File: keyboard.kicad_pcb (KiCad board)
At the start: 2 copper layers, 228.6 x 76.2 mm, 232 parts, among them IC1 ATMEGA32U4, J1 USBMINI_B05, P1 ISP, P2 GPIO Port, Q1 MOS_P, X1 CRYSTAL

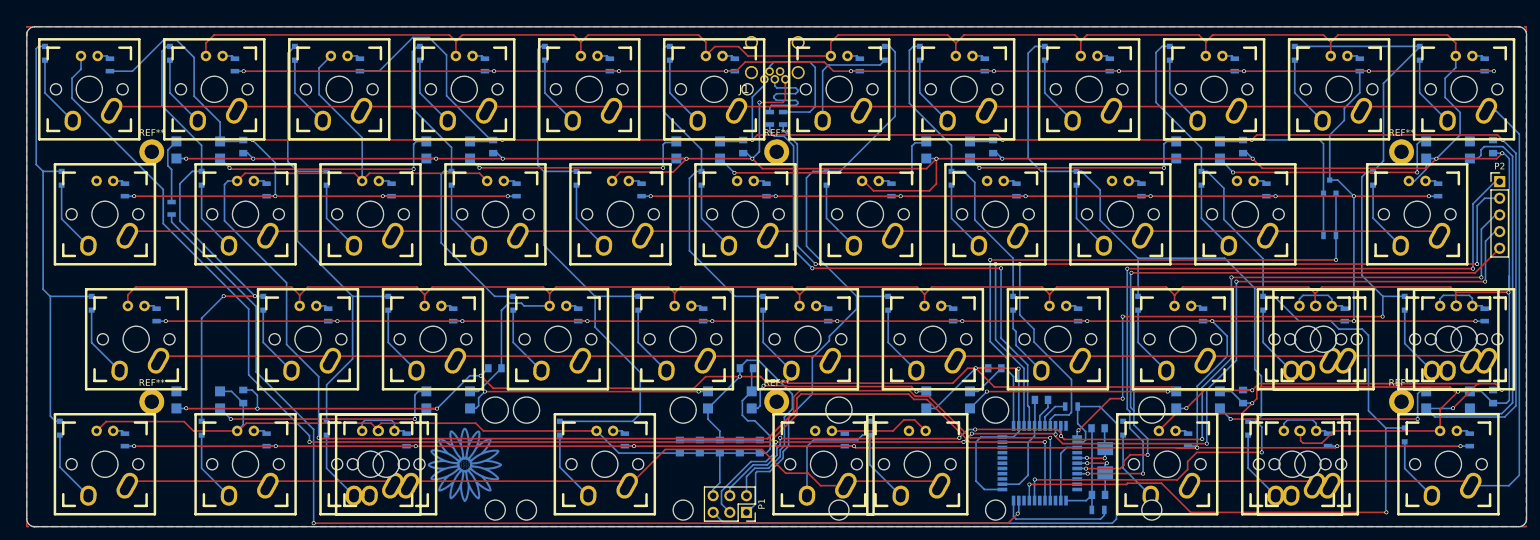
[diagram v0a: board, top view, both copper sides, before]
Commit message: Redesign v0.3
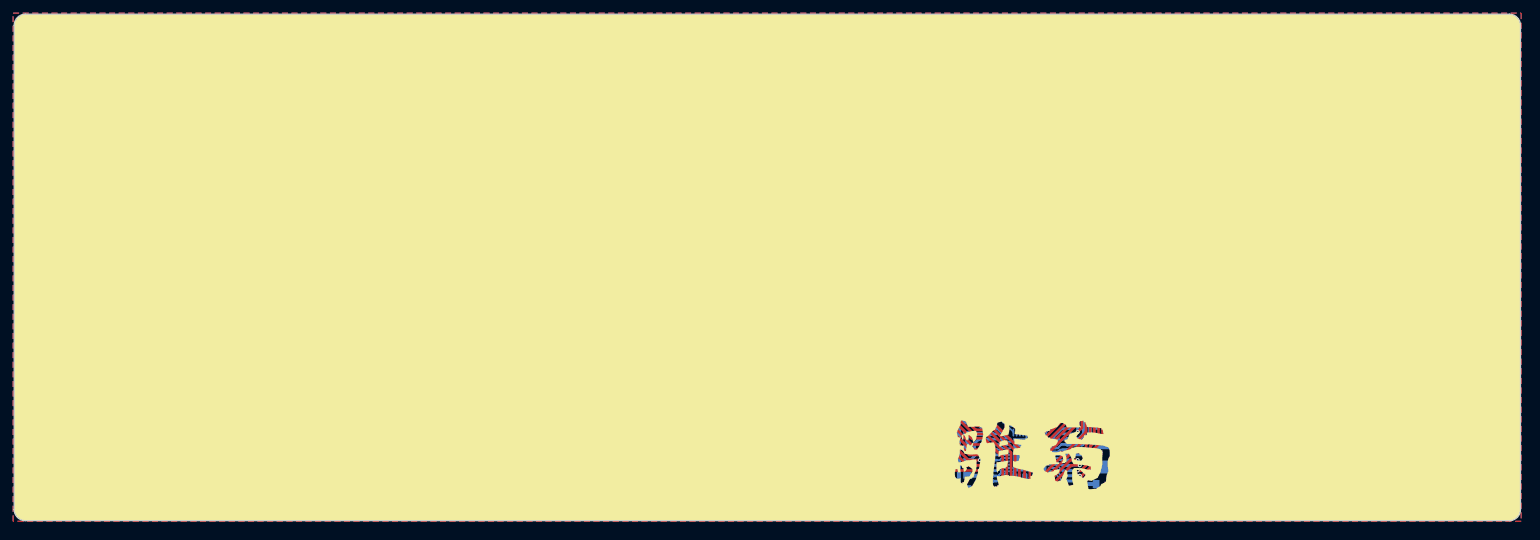
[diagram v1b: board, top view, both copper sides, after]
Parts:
- removed the C17 at (177.5, 82.0)
- removed the C18 at (139.7, 82.0)
- removed C19, C20: 100nF, Capacitors_SMD:C_0805
- removed the G*** at (96.8, 96.8) (x2)
- removed LED331, LED341, LED371, LED391, LED411: LED, mx1a:MX1A-led
- removed LR43: 330R, Resistors_SMD:R_0805
- removed R3: 10K, Resistors_SMD:R_0805
- removed RGBLED10, RGBLED11, RGBLED12, RGBLED9: WS2812B, WS2812B:WS2812B
- removed S321, S331, S361, S401: MX1A, keebs:Mx_Alps_100
- removed ktec-qr: , ktec:ktec-qr
- added ?: , ktec:THX2, B.Cu at (133.3, 95.2)
- added C10: 100nF, capacitors:C_0805, B.Cu at (173.4, 91.1)
- added C4: 100nF, capacitors:C_0805, B.Cu at (173.4, 95.2)
- added DA1: WE05-4RVLCH, diodes:SOT-23-6_Handsoldering, B.Cu at (142.9, 40.0)
- added JP1: JUMPER, passives:Jumper_SMD_2Pads_NC_V, B.Cu at (45.7, 38.1)
- added JP10: JUMPER, passives:Jumper_SMD_2Pads_NC_V, B.Cu at (55.9, 30.8)
- added JP11: JUMPER, passives:Jumper_SMD_2Pads_NC_V, B.Cu at (74.9, 30.8)
- added JP12: JUMPER, passives:Jumper_SMD_2Pads_NC_V, B.Cu at (94.0, 30.8)
- added JP13: JUMPER, passives:Jumper_SMD_2Pads_NC_V, B.Cu at (113.0, 30.8)
- added JP14: JUMPER, passives:Jumper_SMD_2Pads_NC_V, B.Cu at (132.1, 30.8)
- added JP15: JUMPER, passives:Jumper_SMD_2Pads_NC_V, B.Cu at (151.1, 30.8)
- added JP16: JUMPER, passives:Jumper_SMD_2Pads_NC_V, B.Cu at (170.2, 30.8)
- added JP17: JUMPER, passives:Jumper_SMD_2Pads_NC_V, B.Cu at (189.2, 30.8)
- added JP18: JUMPER, passives:Jumper_SMD_2Pads_NC_V, B.Cu at (208.3, 30.8)
- added JP19: JUMPER, passives:Jumper_SMD_2Pads_NC_V, B.Cu at (227.3, 30.8)
- added JP2: JUMPER, passives:Jumper_SMD_2Pads_NC_V, B.Cu at (51.4, 62.9)
- added JP3: JUMPER3, passives:Jumper_SMD_3Pads_NC12, B.Cu at (32.7, 32.1)
- added JP4: JUMPER3, passives:Jumper_SMD_3Pads_NC12, B.Cu at (35.1, 51.1)
- added JP5: JUMPER, passives:Jumper_SMD_2Pads_NC_V, B.Cu at (217.8, 36.8)
- added JP6: JUMPER, passives:Jumper_SMD_2Pads_NC_V, B.Cu at (222.6, 55.9)
- added JP7: JUMPER, passives:Jumper_SMD_2Pads_NC_V, B.Cu at (234.5, 74.9)
- added JP8: JUMPER, passives:Jumper_SMD_2Pads_NC_V, B.Cu at (253.5, 94.0)
- added JP9: JUMPER, passives:Jumper_SMD_2Pads_NC_V, B.Cu at (36.8, 30.8)
- added LED38: LED, leds:MX1A_LED_Polar, F.Cu at (164.3, 95.2)
- added LOGO1: , ktec:Daisy_Logo, B.Cu at (100.0, 94.3)
- added LOGO2: , ktec:Daisy_SilkS, F.Cu at (142.9, 66.7)
- added LR1-2: 330R, resistors:R_0805_NA, B.Cu at (43.8, 34.3)
- added LR12-2: 330R, resistors:R_0805_NA, B.Cu at (46.2, 53.3)
- added P3: GPIO_CLUSTER2, connectors:Socket_Strip_Straight_1x04_Pitch2.54mm, B.Cu at (29.2, 62.9)
- added R6: 4.7K, resistors:R_0805_NA, B.Cu at (34.4, 62.5)
- added R7: 4.7K, resistors:R_0805_NA, B.Cu at (46.5, 62.5)
- added REF**: Via_0.6mm, passives:Via_0.6mm, F.Cu at (127.6, 32.1)
- added SHIELD: Via_0.6mm, passives:Via_0.6mm, F.Cu at (241.6, 78.1)
- added SHIELD: Via_0.6mm, passives:Via_0.6mm, F.Cu at (123.2, 63.2)
- added SHIELD: Via_0.6mm, passives:Via_0.6mm, F.Cu at (70.5, 32.1)
- added SHIELD: Via_0.6mm, passives:Via_0.6mm, F.Cu at (89.5, 32.1)
- added SHIELD: Via_0.6mm, passives:Via_0.6mm, F.Cu at (108.6, 32.1)
- added SHIELD: Via_0.6mm, passives:Via_0.6mm, F.Cu at (165.7, 32.1)
- added SHIELD: Via_0.6mm, passives:Via_0.6mm, F.Cu at (104.1, 63.2)
- added SHIELD: Via_0.6mm, passives:Via_0.6mm, F.Cu at (85.1, 63.2)
- added SHIELD: Via_0.6mm, passives:Via_0.6mm, F.Cu at (66.0, 63.2)
- added SHIELD: Via_0.6mm, passives:Via_0.6mm, F.Cu at (44.1, 63.2)
- added SHIELD: Via_0.6mm, passives:Via_0.6mm, F.Cu at (212.7, 44.8)
- added SHIELD: Via_0.6mm, passives:Via_0.6mm, F.Cu at (193.7, 44.8)
- added SHIELD: Via_0.6mm, passives:Via_0.6mm, F.Cu at (174.6, 44.8)
- added SHIELD: Via_0.6mm, passives:Via_0.6mm, F.Cu at (155.6, 44.8)
- added SHIELD: Via_0.6mm, passives:Via_0.6mm, F.Cu at (117.8, 44.5)
- added SHIELD: Via_0.6mm, passives:Via_0.6mm, F.Cu at (217.5, 97.2)
- added SHIELD: Via_0.6mm, passives:Via_0.6mm, F.Cu at (98.4, 44.8)
- added SHIELD: Via_0.6mm, passives:Via_0.6mm, F.Cu at (79.4, 44.8)
- added SHIELD: Via_0.6mm, passives:Via_0.6mm, F.Cu at (60.3, 44.8)
- added SHIELD: Via_0.6mm, passives:Via_0.6mm, F.Cu at (157.8, 88.6)
- added SHIELD: Via_0.6mm, passives:Via_0.6mm, F.Cu at (208.3, 86.4)
- added SHIELD: Via_0.6mm, passives:Via_0.6mm, F.Cu at (207.3, 93.7)
- added SHIELD: Via_0.6mm, passives:Via_0.6mm, F.Cu at (199.7, 78.7)
- added SHIELD: Via_0.6mm, passives:Via_0.6mm, F.Cu at (157.2, 95.2)
- added SHIELD: Via_0.6mm, passives:Via_0.6mm, F.Cu at (77.2, 97.2)
- added SHIELD: Via_0.6mm, passives:Via_0.6mm, F.Cu at (128.6, 79.4)
- added SHIELD: Via_0.6mm, passives:Via_0.6mm, F.Cu at (151.8, 81.6)
- added SHIELD: Via_0.6mm, passives:Via_0.6mm, F.Cu at (208.3, 74.6)
- added SHIELD: Via_0.6mm, passives:Via_0.6mm, F.Cu at (220.0, 78.1)
- added SHIELD: Via_0.6mm, passives:Via_0.6mm, F.Cu at (218.8, 80.3)
- added SHIELD: Via_0.6mm, passives:Via_0.6mm, F.Cu at (216.2, 80.6)
- added SHIELD: Via_0.6mm, passives:Via_0.6mm, F.Cu at (161.0, 63.2)
- added SHIELD: Via_0.6mm, passives:Via_0.6mm, F.Cu at (218.1, 70.2)
- added SHIELD: Via_0.6mm, passives:Via_0.6mm, F.Cu at (212.4, 71.4)
- added SHIELD: Via_0.6mm, passives:Via_0.6mm, F.Cu at (231.1, 82.5)
- added SHIELD: Via_0.6mm, passives:Via_0.6mm, F.Cu at (239.7, 80.3)
- added SHIELD: Via_0.6mm, passives:Via_0.6mm, F.Cu at (239.4, 70.2)
- added SHIELD: Via_0.6mm, passives:Via_0.6mm, F.Cu at (66.4, 81.6)
- added SHIELD: Via_0.6mm, passives:Via_0.6mm, F.Cu at (122.9, 82.2)
- added SHIELD: Via_0.6mm, passives:Via_0.6mm, F.Cu at (32.7, 62.5)
- added SHIELD: Via_0.6mm, passives:Via_0.6mm, F.Cu at (236.2, 53.3)
- added SHIELD: Via_0.6mm, passives:Via_0.6mm, F.Cu at (48.3, 52.4)
- added SHIELD: Via_0.6mm, passives:Via_0.6mm, F.Cu at (48.9, 55.9)
- added SHIELD: Via_0.6mm, passives:Via_0.6mm, F.Cu at (40.3, 63.2)
- added SHIELD: Via_0.6mm, passives:Via_0.6mm, F.Cu at (57.1, 51.1)
- added SHIELD: Via_0.6mm, passives:Via_0.6mm, F.Cu at (114.3, 43.5)
- added SHIELD: Via_0.6mm, passives:Via_0.6mm, F.Cu at (180.7, 78.7)
- added SHIELD: Via_0.6mm, passives:Via_0.6mm, F.Cu at (189.9, 74.3)
- added SHIELD: Via_0.6mm, passives:Via_0.6mm, F.Cu at (40.6, 85.1)
- added SHIELD: Via_0.6mm, passives:Via_0.6mm, F.Cu at (203.5, 102.2)
- added SHIELD: Via_0.6mm, passives:Via_0.6mm, F.Cu at (215.9, 89.2)
- added SHIELD: Via_0.6mm, passives:Via_0.6mm, F.Cu at (247.3, 85.7)
- added SHIELD: Via_0.6mm, passives:Via_0.6mm, F.Cu at (161.6, 78.7)
- added SHIELD: Via_0.6mm, passives:Via_0.6mm, F.Cu at (84.8, 82.5)
- added SHIELD: Via_0.6mm, passives:Via_0.6mm, F.Cu at (73.7, 89.2)
- added SHIELD: Via_0.6mm, passives:Via_0.6mm, F.Cu at (43.5, 43.5)
- added SHIELD: Via_0.6mm, passives:Via_0.6mm, F.Cu at (39.1, 47.6)
- added SHIELD: Via_0.6mm, passives:Via_0.6mm, F.Cu at (58.7, 76.2)
- added SHIELD: Via_0.6mm, passives:Via_0.6mm, F.Cu at (100.0, 76.2)
- added SHIELD: Via_0.6mm, passives:Via_0.6mm, F.Cu at (244.8, 63.2)
- added SHIELD: Via_0.6mm, passives:Via_0.6mm, F.Cu at (119.1, 76.2)
- added SHIELD: Via_0.6mm, passives:Via_0.6mm, F.Cu at (138.1, 76.2)
- added SHIELD: Via_0.6mm, passives:Via_0.6mm, F.Cu at (134.0, 87.9)
- added SHIELD: Via_0.6mm, passives:Via_0.6mm, F.Cu at (109.9, 88.6)
- added SHIELD: Via_0.6mm, passives:Via_0.6mm, F.Cu at (254.0, 101.9)
- added SHIELD: Via_0.6mm, passives:Via_0.6mm, F.Cu at (31.8, 101.9)
- added SHIELD: Via_0.6mm, passives:Via_0.6mm, F.Cu at (144.8, 61.3)
- added SHIELD: Via_0.6mm, passives:Via_0.6mm, F.Cu at (138.1, 63.5)
- added SHIELD: Via_0.6mm, passives:Via_0.6mm, F.Cu at (161.0, 70.2)
- added SHIELD: Via_0.6mm, passives:Via_0.6mm, F.Cu at (157.2, 62.9)
- added SHIELD: Via_0.6mm, passives:Via_0.6mm, F.Cu at (199.4, 63.2)
- added SHIELD: Via_0.6mm, passives:Via_0.6mm, F.Cu at (218.4, 63.2)
- added SHIELD: Via_0.6mm, passives:Via_0.6mm, F.Cu at (222.6, 61.6)
- added SHIELD: Via_0.6mm, passives:Via_0.6mm, F.Cu at (227.3, 56.8)
- added SHIELD: Via_0.6mm, passives:Via_0.6mm, F.Cu at (185.7, 57.1)
- added SHIELD: Via_0.6mm, passives:Via_0.6mm, F.Cu at (166.7, 57.1)
- added SHIELD: Via_0.6mm, passives:Via_0.6mm, F.Cu at (141.9, 70.2)
- added SHIELD: Via_0.6mm, passives:Via_0.6mm, F.Cu at (34.6, 73.3)
- added SHIELD: Via_0.6mm, passives:Via_0.6mm, F.Cu at (32.7, 54.3)
- added SHIELD: Via_0.6mm, passives:Via_0.6mm, F.Cu at (56.5, 61.0)
- added SHIELD: Via_0.6mm, passives:Via_0.6mm, F.Cu at (71.4, 57.1)
- added SHIELD: Via_0.6mm, passives:Via_0.6mm, F.Cu at (180.3, 63.2)
- added SHIELD: Via_0.6mm, passives:Via_0.6mm, F.Cu at (90.5, 57.1)
- added SHIELD: Via_0.6mm, passives:Via_0.6mm, F.Cu at (109.5, 57.1)
- added SHIELD: Via_0.6mm, passives:Via_0.6mm, F.Cu at (128.6, 57.1)
- added SHIELD: Via_0.6mm, passives:Via_0.6mm, F.Cu at (139.1, 42.5)
- added SHIELD: Via_0.6mm, passives:Via_0.6mm, F.Cu at (136.5, 45.1)
- added SHIELD: Via_0.6mm, passives:Via_0.6mm, F.Cu at (146.7, 42.5)
- added SHIELD: Via_0.6mm, passives:Via_0.6mm, F.Cu at (113.0, 51.1)
- added SHIELD: Via_0.6mm, passives:Via_0.6mm, F.Cu at (132.1, 51.1)
- added SHIELD: Via_0.6mm, passives:Via_0.6mm, F.Cu at (246.4, 48.6)
- added SHIELD: Via_0.6mm, passives:Via_0.6mm, F.Cu at (253.4, 56.2)
- added SHIELD: Via_0.6mm, passives:Via_0.6mm, F.Cu at (142.2, 63.2)
- added SHIELD: Via_0.6mm, passives:Via_0.6mm, F.Cu at (224.8, 51.1)
- added SHIELD: Via_0.6mm, passives:Via_0.6mm, F.Cu at (234.9, 44.1)
- added SHIELD: Via_0.6mm, passives:Via_0.6mm, F.Cu at (189.2, 51.1)
- added SHIELD: Via_0.6mm, passives:Via_0.6mm, F.Cu at (104.8, 38.1)
- added SHIELD: Via_0.6mm, passives:Via_0.6mm, F.Cu at (161.9, 38.1)
- added SHIELD: Via_0.6mm, passives:Via_0.6mm, F.Cu at (123.8, 38.1)
- added SHIELD: Via_0.6mm, passives:Via_0.6mm, F.Cu at (222.9, 32.1)
- added SHIELD: Via_0.6mm, passives:Via_0.6mm, F.Cu at (203.8, 32.1)
- added SHIELD: Via_0.6mm, passives:Via_0.6mm, F.Cu at (184.8, 32.1)
- added SHIELD: Via_0.6mm, passives:Via_0.6mm, F.Cu at (51.4, 32.1)
- C1, C2, C3: footprint Capacitors_SMD:C_0805 -> capacitors:C_0805
- C11: renamed from C9; footprint Capacitors_SMD:C_0805 -> capacitors:C_0805_V2
- C12: renamed from C10; footprint Capacitors_SMD:C_0805 -> capacitors:C_0805_V2
- C13: renamed from C11; footprint Capacitors_SMD:C_0805 -> capacitors:C_0805_V2
- C14: renamed from C12; footprint Capacitors_SMD:C_0805 -> capacitors:C_0805_V1
- C15: renamed from C13; footprint Capacitors_SMD:C_0805 -> capacitors:C_0805_V1
- C16: renamed from C14; footprint Capacitors_SMD:C_0805 -> capacitors:C_0805_V1
- C17: renamed from C15; footprint Capacitors_SMD:C_0805 -> capacitors:C_0805_V1
- C18: renamed from C16; footprint Capacitors_SMD:C_0805 -> capacitors:C_0805_V2
- C5: renamed from C8; footprint Capacitors_SMD:C_0805 -> capacitors:C_0805
- C6: renamed from C4; footprint Capacitors_SMD:C_0805 -> capacitors:C_0805
- C7: renamed from C5; footprint Capacitors_SMD:C_0805 -> capacitors:C_0805
- C8: renamed from C6; footprint Capacitors_SMD:C_0805 -> capacitors:C_0805
- C9: renamed from C7; footprint Capacitors_SMD:C_0805 -> capacitors:C_0805
- D1, D10, D11, D12, D13, D14, D15, D16, D17, D18, D19, D2, D20, D21, D22, D23, D24, D25, D26, D27, D28, D29, D3, D30, D31, D32, D33, D34, D35, D36, D37, D38, D39, D4, D40, D41, D42, D5, D6, D7, D8, D9: footprint Diodes_SMD:D_0805 -> diodes:D_0805_V2
- J1: value USBMINI_B05 -> USB_MINI-B; footprint USB:DX_USB -> connectors:USB_MINI-B
- LED1, LED10, LED11, LED12, LED13, LED14, LED15, LED16, LED17, LED18, LED19, LED2, LED20, LED21, LED22, LED23, LED24, LED25, LED26, LED27, LED28, LED29, LED3, LED30, LED31, LED34, LED35, LED37, LED39, LED4, LED41, LED42, LED5, LED6, LED7, LED8, LED9: footprint mx1a:MX1A-led -> leds:MX1A_LED_Polar
- LED32, LED33, LED36, LED40: footprint mx1a:MX1A-led -> leds:MX1A_LED_Polar_Dual
- LED38_625: renamed from LED38; footprint mx1a:MX1A-led -> leds:MX1A_LED_Polar
- LR1, LR10, LR11, LR12, LR13, LR14, LR15, LR16, LR17, LR18, LR19, LR2, LR20, LR21, LR22, LR23, LR24, LR25, LR26, LR27, LR28, LR29, LR3, LR30, LR31, LR32, LR33, LR34, LR35, LR36, LR37, LR38, LR39, LR4, LR40, LR41, LR42, LR5, LR6, LR7, LR8, LR9, R1, R2: footprint Resistors_SMD:R_0805 -> resistors:R_0805_V1
- P1: footprint Socket_Strips:Socket_Strip_Straight_2x03_Pitch2.54mm -> connectors:Socket_Strip_Straight_1x06_Pitch2.54mm; moved to B.Cu
- P2: value GPIO Port -> GPIO_CLUSTER1; footprint Socket_Strips:Socket_Strip_Straight_1x05_Pitch2.54mm -> connectors:Socket_Strip_Straight_2x04_Pitch2.54mm; moved to B.Cu
- Q1: footprint SI2305:SOT-23 -> transistors:SOT-23
- R4, R5: footprint Resistors_SMD:R_0805 -> resistors:R_0805
- RGBLED1, RGBLED2, RGBLED3, RGBLED4, RGBLED5, RGBLED6, RGBLED7, RGBLED8: footprint WS2812B:WS2812B -> leds:WS2812B
- SW1: renamed from S1; footprint keebs:Mx_Alps_100 -> switches:Mx_Alps_100_NoFSilk
- SW10: renamed from S10; footprint keebs:Mx_Alps_100 -> switches:Mx_Alps_100_NoFSilk
- SW11: renamed from S11; footprint keebs:Mx_Alps_100 -> switches:Mx_Alps_100_NoFSilk
- SW12: renamed from S12; footprint keebs:Mx_Alps_100 -> switches:Mx_Alps_125_NoFSilk
- SW13: renamed from S13; footprint keebs:Mx_Alps_100 -> switches:Mx_Alps_100_NoFSilk
- SW14: renamed from S14; footprint keebs:Mx_Alps_100 -> switches:Mx_Alps_100_NoFSilk
- SW15: renamed from S15; footprint keebs:Mx_Alps_100 -> switches:Mx_Alps_100_NoFSilk
- SW16: renamed from S16; footprint keebs:Mx_Alps_100 -> switches:Mx_Alps_100_NoFSilk
- SW17: renamed from S17; footprint keebs:Mx_Alps_100 -> switches:Mx_Alps_100_NoFSilk
- SW18: renamed from S18; footprint keebs:Mx_Alps_100 -> switches:Mx_Alps_100_NoFSilk
- SW19: renamed from S19; footprint keebs:Mx_Alps_100 -> switches:Mx_Alps_100_NoFSilk
- SW2: renamed from S2; footprint keebs:Mx_Alps_100 -> switches:Mx_Alps_100_NoFSilk
- SW20: renamed from S20; footprint keebs:Mx_Alps_100 -> switches:Mx_Alps_100_NoFSilk
- SW21: renamed from S21; footprint keebs:Mx_Alps_100 -> switches:Mx_Alps_100_NoFSilk
- SW22: renamed from S22; footprint keebs:Mx_Alps_100 -> switches:Mx_Alps_175_NoFSilk
- SW23: renamed from S23; footprint keebs:Mx_Alps_100 -> switches:Mx_Alps_175_NoFSilk
- SW24: renamed from S24; footprint keebs:Mx_Alps_100 -> switches:Mx_Alps_100_NoFSilk
- SW25: renamed from S25; footprint keebs:Mx_Alps_100 -> switches:Mx_Alps_100_NoFSilk
- SW26: renamed from S26; footprint keebs:Mx_Alps_100 -> switches:Mx_Alps_100_NoFSilk
- SW27: renamed from S27; footprint keebs:Mx_Alps_100 -> switches:Mx_Alps_100_NoFSilk
- SW28: renamed from S28; footprint keebs:Mx_Alps_100 -> switches:Mx_Alps_100_NoFSilk
- SW29: renamed from S29; footprint keebs:Mx_Alps_100 -> switches:Mx_Alps_100_NoFSilk
- SW3: renamed from S3; footprint keebs:Mx_Alps_100 -> switches:Mx_Alps_100_NoFSilk
- SW30: renamed from S30; footprint keebs:Mx_Alps_100 -> switches:Mx_Alps_100_NoFSilk
- SW31: renamed from S31; footprint keebs:Mx_Alps_100 -> switches:Mx_Alps_100_NoFSilk
- SW32: renamed from S32; footprint keebs:Mx_Alps_100 -> switches:Mx_Alps_100_Dual_NoFSilk
- SW33: renamed from S33; footprint keebs:Mx_Alps_100 -> switches:Mx_Alps_100_Dual_NoFSilk
- SW34: renamed from S34; footprint keebs:Mx_Alps_100 -> switches:Mx_Alps_125_NoFSilk
- SW35: renamed from S35; footprint keebs:Mx_Alps_100 -> switches:Mx_Alps_100_NoFSilk
- SW36: renamed from S36; footprint keebs:Mx_Alps_100 -> switches:Mx_Alps_100_Dual_NoFSilk
- SW37: renamed from S37; footprint keebs:Mx_Alps_225 -> switches:Mx_Alps_225_NoFSilk
- SW38: renamed from S381; footprint keebs:Mx_Alps_275 -> switches:Mx_Alps_275_NoFSilk
- SW38_625: renamed from S38; footprint keebs:Mx_Alps_625 -> switches:Mx_Alps_625_NoFSilk
- SW39: renamed from S39; footprint keebs:Mx_Alps_100 -> switches:Mx_Alps_100_NoFSilk
- SW4: renamed from S4; footprint keebs:Mx_Alps_100 -> switches:Mx_Alps_100_NoFSilk
- SW40: renamed from S40; footprint keebs:Mx_Alps_100 -> switches:Mx_Alps_100_Dual_NoFSilk
- SW41: renamed from S41; footprint keebs:Mx_Alps_100 -> switches:Mx_Alps_125_NoFSilk
- SW42: renamed from S42; footprint keebs:Mx_Alps_100 -> switches:Mx_Alps_100_NoFSilk
- SW5: renamed from S5; footprint keebs:Mx_Alps_100 -> switches:Mx_Alps_100_NoFSilk
- SW6: renamed from S6; footprint keebs:Mx_Alps_100 -> switches:Mx_Alps_100_NoFSilk
- SW7: renamed from S7; footprint keebs:Mx_Alps_100 -> switches:Mx_Alps_100_NoFSilk
- SW8: renamed from S8; footprint keebs:Mx_Alps_100 -> switches:Mx_Alps_100_NoFSilk
- SW9: renamed from S9; footprint keebs:Mx_Alps_100 -> switches:Mx_Alps_100_NoFSilk
- U1: renamed from IC1; footprint Housings_QFP:TQFP-44_10x10mm_Pitch0.8mm -> housings:TQFP44+QFN44
- moved LED34 209.3 mm to (40.5, 95.2)
- moved LR34 206.8 mm to (46.2, 91.4), turned to 270 degrees
- moved LED23 197.5 mm to (45.2, 76.2)
- moved LR23 194.9 mm to (51.0, 72.4), turned to 270 degrees
- moved LR11 190.5 mm to (234.3, 34.3), turned to 270 degrees
- moved LED11 187.8 mm to (228.6, 38.1)
- moved Q1 177.2 mm to (51.4, 57.1)
- moved R4 177.2 mm to (51.4, 60.3)
- moved RGBLED1 118.1 mm to (168.3, 85.7), turned to 0 degrees
- moved C11 106.7 mm to (162.9, 85.7)
- moved C14 105.2 mm to (72.1, 47.6), turned to 270 degrees
- moved RGBLED4 103.8 mm to (66.7, 47.6)
- moved C15 92.5 mm to (122.9, 47.6), turned to 270 degrees
- moved RGBLED5 91.1 mm to (117.5, 47.6)
- moved C16 90.6 mm to (162.9, 47.6), turned to 270 degrees
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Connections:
- net /~Res renamed /~RESET
- C11 pad 1: GND -> VCC
- C11 pad 2: VCC -> GND
- C12 pad 1: GND -> VCC
- C12 pad 2: VCC -> GND
- C13 pad 1: GND -> VCC
- C13 pad 2: VCC -> GND
- C14 pad 1: GND -> VCC
- C14 pad 2: VCC -> GND
- C15 pad 1: GND -> VCC
- C15 pad 2: VCC -> GND
- C16 pad 1: GND -> VCC
- C16 pad 2: VCC -> GND
- C17 pad 1: GND -> VCC
- C17 pad 2: VCC -> GND
- C18 pad 1: GND -> VCC
- C18 pad 2: VCC -> GND
- D1 pad 1: /Col0 -> Net-(D1-Pad1)
- D1 pad 2: Net-(D1-Pad2) -> /matrix/Row0
- D10 pad 1: /Col9 -> Net-(D10-Pad1)
- D10 pad 2: Net-(D10-Pad2) -> /matrix/Row0
- D11 pad 1: /Col10 -> Net-(D11-Pad1)
- D11 pad 2: Net-(D11-Pad2) -> /matrix/Row0
- D12 pad 1: /Col0 -> Net-(D12-Pad1)
- D12 pad 2: Net-(D12-Pad2) -> /matrix/Row1
- D13 pad 1: /Col1 -> Net-(D13-Pad1)
- D13 pad 2: Net-(D13-Pad2) -> /matrix/Row1
- D14 pad 1: /Col2 -> Net-(D14-Pad1)
- D14 pad 2: Net-(D14-Pad2) -> /matrix/Row1
- D15 pad 1: /Col3 -> Net-(D15-Pad1)
- D15 pad 2: Net-(D15-Pad2) -> /matrix/Row1
- D16 pad 1: /Col4 -> Net-(D16-Pad1)
- D16 pad 2: Net-(D16-Pad2) -> /matrix/Row1
- D17 pad 1: /Col5 -> Net-(D17-Pad1)
- D17 pad 2: Net-(D17-Pad2) -> /matrix/Row1
- D18 pad 1: /Col6 -> Net-(D18-Pad1)
- D18 pad 2: Net-(D18-Pad2) -> /matrix/Row1
- D19 pad 1: /Col7 -> Net-(D19-Pad1)
- D19 pad 2: Net-(D19-Pad2) -> /matrix/Row1
- D2 pad 1: /Col1 -> Net-(D2-Pad1)
- D2 pad 2: Net-(D2-Pad2) -> /matrix/Row0
- D20 pad 1: /Col8 -> Net-(D20-Pad1)
- D20 pad 2: Net-(D20-Pad2) -> /matrix/Row1
- D21 pad 1: /Col9 -> Net-(D21-Pad1)
- D21 pad 2: Net-(D21-Pad2) -> /matrix/Row1
- D22 pad 1: /Col10 -> Net-(D22-Pad1)
- D22 pad 2: Net-(D22-Pad2) -> /matrix/Row1
- D23 pad 1: /Col0 -> Net-(D23-Pad1)
- D23 pad 2: Net-(D23-Pad2) -> /matrix/Row2
- D24 pad 1: /Col1 -> Net-(D24-Pad1)
- D24 pad 2: Net-(D24-Pad2) -> /matrix/Row2
- D25 pad 1: /Col2 -> Net-(D25-Pad1)
- D25 pad 2: Net-(D25-Pad2) -> /matrix/Row2
- D26 pad 1: /Col3 -> Net-(D26-Pad1)
- D26 pad 2: Net-(D26-Pad2) -> /matrix/Row2
- D27 pad 1: /Col4 -> Net-(D27-Pad1)
- D27 pad 2: Net-(D27-Pad2) -> /matrix/Row2
- D28 pad 1: /Col5 -> Net-(D28-Pad1)
- D28 pad 2: Net-(D28-Pad2) -> /matrix/Row2
- D29 pad 1: /Col6 -> Net-(D29-Pad1)
- D29 pad 2: Net-(D29-Pad2) -> /matrix/Row2
- D3 pad 1: /Col2 -> Net-(D3-Pad1)
- D3 pad 2: Net-(D3-Pad2) -> /matrix/Row0
- D30 pad 1: /Col7 -> Net-(D30-Pad1)
- D30 pad 2: Net-(D30-Pad2) -> /matrix/Row2
- D31 pad 1: /Col8 -> Net-(D31-Pad1)
- D31 pad 2: Net-(D31-Pad2) -> /matrix/Row2
- D32 pad 1: /Col9 -> Net-(D32-Pad1)
- D32 pad 2: Net-(D32-Pad2) -> /matrix/Row2
- D33 pad 1: /Col10 -> Net-(D33-Pad1)
- D33 pad 2: Net-(D33-Pad2) -> /matrix/Row2
- D34 pad 1: /Col0 -> Net-(D34-Pad1)
- D34 pad 2: Net-(D34-Pad2) -> /matrix/Row3
- D35 pad 1: /Col1 -> Net-(D35-Pad1)
- D35 pad 2: Net-(D35-Pad2) -> /matrix/Row3
- D36 pad 1: /Col2 -> Net-(D36-Pad1)
- D36 pad 2: Net-(D36-Pad2) -> /matrix/Row3
- D37 pad 1: /Col4 -> Net-(D37-Pad1)
- D37 pad 2: Net-(D37-Pad2) -> /matrix/Row3
- D38 pad 1: /Col5 -> Net-(D38-Pad1)
- D38 pad 2: Net-(D38-Pad2) -> /matrix/Row3
- D39 pad 1: /Col7 -> Net-(D39-Pad1)
- D39 pad 2: Net-(D39-Pad2) -> /matrix/Row3
- D4 pad 1: /Col3 -> Net-(D4-Pad1)
- D4 pad 2: Net-(D4-Pad2) -> /matrix/Row0
- D40 pad 1: /Col8 -> Net-(D40-Pad1)
- D40 pad 2: Net-(D40-Pad2) -> /matrix/Row3
- D41 pad 1: /Col9 -> Net-(D41-Pad1)
- D41 pad 2: Net-(D41-Pad2) -> /matrix/Row3
- D42 pad 1: /Col10 -> Net-(D42-Pad1)
- D42 pad 2: Net-(D42-Pad2) -> /matrix/Row3
- D5 pad 1: /Col4 -> Net-(D5-Pad1)
- D5 pad 2: Net-(D5-Pad2) -> /matrix/Row0
- D6 pad 1: /Col5 -> Net-(D6-Pad1)
- D6 pad 2: Net-(D6-Pad2) -> /matrix/Row0
- D7 pad 1: /Col6 -> Net-(D7-Pad1)
- D7 pad 2: Net-(D7-Pad2) -> /matrix/Row0
- D8 pad 1: /Col7 -> Net-(D8-Pad1)
- D8 pad 2: Net-(D8-Pad2) -> /matrix/Row0
- D9 pad 1: /Col8 -> Net-(D9-Pad1)
- D9 pad 2: Net-(D9-Pad2) -> /matrix/Row0
- LED1 pad 1: Net-(LED1-Pad1) -> Net-(JP3-Pad2)
- LED1 pad 2: GND -> Net-(LED1-Pad2)
- LED10 pad 1: Net-(LED10-Pad1) -> /led/LCol9
- LED10 pad 2: GND -> Net-(LED10-Pad2)
- LED11 pad 1: Net-(LED11-Pad1) -> /led/LCol10
- LED11 pad 2: /Caps -> Net-(LED11-Pad2)
- LED12 pad 1: Net-(LED12-Pad1) -> Net-(JP4-Pad2)
- LED12 pad 2: /ESC -> Net-(LED12-Pad2)
- LED13 pad 1: Net-(LED13-Pad1) -> /led/LCol1
- LED13 pad 2: /WASD -> Net-(LED13-Pad2)
- LED14 pad 1: Net-(LED14-Pad1) -> /led/LCol2
- LED14 pad 2: /WASD -> Net-(LED14-Pad2)
- LED15 pad 1: Net-(LED15-Pad1) -> /led/LCol3
- LED15 pad 2: /WASD -> Net-(LED15-Pad2)
- LED16 pad 1: Net-(LED16-Pad1) -> /led/LCol4
- LED16 pad 2: /WASD -> Net-(LED16-Pad2)
- LED17 pad 1: Net-(LED17-Pad1) -> /led/LCol5
- LED17 pad 2: GND -> Net-(LED17-Pad2)
- LED18 pad 1: Net-(LED18-Pad1) -> /led/LCol6
- LED18 pad 2: GND -> Net-(LED18-Pad2)
- LED19 pad 1: Net-(LED19-Pad1) -> /led/LCol7
- LED19 pad 2: GND -> Net-(LED19-Pad2)
- LED2 pad 1: Net-(LED2-Pad1) -> /led/LCol1
- LED2 pad 2: GND -> Net-(LED2-Pad2)
- LED20 pad 1: Net-(LED20-Pad1) -> /led/LCol8
- LED20 pad 2: GND -> Net-(LED20-Pad2)
- LED21 pad 1: Net-(LED21-Pad1) -> /led/LCol9
- LED21 pad 2: GND -> Net-(LED21-Pad2)
- LED22 pad 1: Net-(LED22-Pad1) -> /led/LCol10
- LED22 pad 2: GND -> Net-(LED22-Pad2)
- LED23 pad 1: Net-(LED23-Pad1) -> /led/LCol0
- LED23 pad 2: GND -> Net-(LED23-Pad2)
- LED24 pad 1: Net-(LED24-Pad1) -> /led/LCol1
- LED24 pad 2: GND -> Net-(LED24-Pad2)
- LED25 pad 1: Net-(LED25-Pad1) -> /led/LCol2
- LED25 pad 2: GND -> Net-(LED25-Pad2)
- LED26 pad 1: Net-(LED26-Pad1) -> /led/LCol3
- LED26 pad 2: GND -> Net-(LED26-Pad2)
- LED27 pad 1: Net-(LED27-Pad1) -> /led/LCol4
- LED27 pad 2: GND -> Net-(LED27-Pad2)
- LED28 pad 1: Net-(LED28-Pad1) -> /led/LCol5
- LED28 pad 2: GND -> Net-(LED28-Pad2)
- LED29 pad 1: Net-(LED29-Pad1) -> /led/LCol6
- LED29 pad 2: GND -> Net-(LED29-Pad2)
- LED3 pad 1: Net-(LED3-Pad1) -> /led/LCol2
- LED3 pad 2: GND -> Net-(LED3-Pad2)
- LED30 pad 1: Net-(LED30-Pad1) -> /led/LCol7
- LED30 pad 2: GND -> Net-(LED30-Pad2)
- LED31 pad 1: Net-(LED31-Pad1) -> /led/LCol8
- LED31 pad 2: GND -> Net-(LED31-Pad2)
- LED32 pad 1: Net-(LED32-Pad1) -> /led/LCol9
- LED32 pad 2: GND -> Net-(LED32-Pad2)
- LED33 pad 1: Net-(LED33-Pad1) -> /led/LCol10
- LED33 pad 2: GND -> Net-(LED33-Pad2)
- LED34 pad 1: Net-(LED34-Pad1) -> /led/LCol0
- LED34 pad 2: GND -> Net-(LED34-Pad2)
- LED35 pad 1: Net-(LED35-Pad1) -> /led/LCol1
- LED35 pad 2: GND -> Net-(LED35-Pad2)
- LED36 pad 1: Net-(LED36-Pad1) -> /led/LCol2
- LED36 pad 2: GND -> Net-(LED36-Pad2)
- LED37 pad 1: Net-(LED37-Pad1) -> /led/LCol4
- LED37 pad 2: GND -> Net-(LED37-Pad2)
- LED38_625 pad 1: Net-(LED38-Pad1) -> /led/LCol5
- LED38_625 pad 2: GND -> Net-(LED38-Pad2)
- LED39 pad 1: Net-(LED39-Pad1) -> /led/LCol7
- LED39 pad 2: GND -> Net-(LED39-Pad2)
- LED4 pad 1: Net-(LED4-Pad1) -> /led/LCol3
- LED4 pad 2: GND -> Net-(LED4-Pad2)
- LED40 pad 1: Net-(LED40-Pad1) -> /led/LCol8
- LED40 pad 2: GND -> Net-(LED40-Pad2)
- LED41 pad 1: Net-(LED41-Pad1) -> /led/LCol9
- LED41 pad 2: GND -> Net-(LED41-Pad2)
- LED42 pad 1: Net-(LED42-Pad1) -> /led/LCol10
- LED42 pad 2: GND -> Net-(LED42-Pad2)
- LED5 pad 1: Net-(LED5-Pad1) -> /led/LCol4
- LED5 pad 2: GND -> Net-(LED5-Pad2)
- LED6 pad 1: Net-(LED6-Pad1) -> /led/LCol5
- LED6 pad 2: GND -> Net-(LED6-Pad2)
- LED7 pad 1: Net-(LED7-Pad1) -> /led/LCol6
- LED7 pad 2: GND -> Net-(LED7-Pad2)
- LED8 pad 1: Net-(LED8-Pad1) -> /led/LCol7
- LED8 pad 2: GND -> Net-(LED8-Pad2)
- LED9 pad 1: Net-(LED9-Pad1) -> /led/LCol8
- LED9 pad 2: GND -> Net-(LED9-Pad2)
- LR1 pad 1: /led/LRow0 -> Net-(LED1-Pad2)
- LR1 pad 2: Net-(LED1-Pad1) -> /led/Esc
- LR10 pad 1: /led/LRow0 -> Net-(LED10-Pad2)
- LR10 pad 2: Net-(LED10-Pad1) -> /led/LRow0
- LR11 pad 1: VCC -> Net-(LED11-Pad2)
- LR11 pad 2: Net-(LED11-Pad1) -> /led/LRow0
- LR12 pad 1: VCC -> Net-(LED12-Pad2)
- LR12 pad 2: Net-(LED12-Pad1) -> /led/CapsLock
- LR13 pad 1: VCC -> Net-(LED13-Pad2)
- LR13 pad 2: Net-(LED13-Pad1) -> /led/LRow1
- LR14 pad 1: VCC -> Net-(LED14-Pad2)
- LR14 pad 2: Net-(LED14-Pad1) -> /led/LRow1
- LR15 pad 1: VCC -> Net-(LED15-Pad2)
- LR15 pad 2: Net-(LED15-Pad1) -> /led/LRow1
- LR16 pad 1: VCC -> Net-(LED16-Pad2)
- LR16 pad 2: Net-(LED16-Pad1) -> /led/LRow1
- LR17 pad 1: /led/LRow0 -> Net-(LED17-Pad2)
- LR17 pad 2: Net-(LED17-Pad1) -> /led/LRow1
- LR18 pad 1: /led/LRow0 -> Net-(LED18-Pad2)
- LR18 pad 2: Net-(LED18-Pad1) -> /led/LRow1
- LR19 pad 1: /led/LRow0 -> Net-(LED19-Pad2)
- LR19 pad 2: Net-(LED19-Pad1) -> /led/LRow1
- LR2 pad 1: /led/LRow0 -> Net-(LED2-Pad2)
- LR2 pad 2: Net-(LED2-Pad1) -> /led/LRow0
- LR20 pad 1: /led/LRow0 -> Net-(LED20-Pad2)
- LR20 pad 2: Net-(LED20-Pad1) -> /led/LRow1
- LR21 pad 1: /led/LRow0 -> Net-(LED21-Pad2)
- LR21 pad 2: Net-(LED21-Pad1) -> /led/LRow1
- LR22 pad 1: /led/LRow0 -> Net-(LED22-Pad2)
- LR22 pad 2: Net-(LED22-Pad1) -> /led/LRow1
- LR23 pad 1: /led/LRow0 -> Net-(LED23-Pad2)
- LR23 pad 2: Net-(LED23-Pad1) -> /led/LRow2
- LR24 pad 1: /led/LRow0 -> Net-(LED24-Pad2)
- LR24 pad 2: Net-(LED24-Pad1) -> /led/LRow2
- LR25 pad 1: /led/LRow0 -> Net-(LED25-Pad2)
- LR25 pad 2: Net-(LED25-Pad1) -> /led/LRow2
- LR26 pad 1: /led/LRow0 -> Net-(LED26-Pad2)
- LR26 pad 2: Net-(LED26-Pad1) -> /led/LRow2
- LR27 pad 1: /led/LRow0 -> Net-(LED27-Pad2)
- LR27 pad 2: Net-(LED27-Pad1) -> /led/LRow2
- LR28 pad 1: /led/LRow0 -> Net-(LED28-Pad2)
- LR28 pad 2: Net-(LED28-Pad1) -> /led/LRow2
- LR29 pad 1: /led/LRow0 -> Net-(LED29-Pad2)
- LR29 pad 2: Net-(LED29-Pad1) -> /led/LRow2
- LR3 pad 1: /led/LRow0 -> Net-(LED3-Pad2)
- LR3 pad 2: Net-(LED3-Pad1) -> /led/LRow0
- LR30 pad 1: /led/LRow0 -> Net-(LED30-Pad2)
- LR30 pad 2: Net-(LED30-Pad1) -> /led/LRow2
- LR31 pad 1: /led/LRow0 -> Net-(LED31-Pad2)
- LR31 pad 2: Net-(LED31-Pad1) -> /led/LRow2
- LR32 pad 1: /led/LRow0 -> Net-(LED32-Pad2)
- LR32 pad 2: Net-(LED32-Pad1) -> /led/LRow2
- LR33 pad 1: /led/LRow0 -> Net-(LED33-Pad2)
- LR33 pad 2: Net-(LED33-Pad1) -> /led/LRow2
- LR34 pad 1: /led/LRow0 -> Net-(LED34-Pad2)
- LR34 pad 2: Net-(LED34-Pad1) -> /led/LRow3
- LR35 pad 1: /led/LRow0 -> Net-(LED35-Pad2)
- LR35 pad 2: Net-(LED35-Pad1) -> /led/LRow3
- LR36 pad 1: /led/LRow0 -> Net-(LED36-Pad2)
- LR36 pad 2: Net-(LED36-Pad1) -> /led/LRow3
- LR37 pad 1: /led/LRow0 -> Net-(LED37-Pad2)
- LR37 pad 2: Net-(LED37-Pad1) -> /led/LRow3
- LR38 pad 1: /led/LRow0 -> Net-(LED38-Pad2)
- LR38 pad 2: Net-(LED38-Pad1) -> /led/LRow3
- LR39 pad 1: /led/LRow0 -> Net-(LED39-Pad2)
- LR39 pad 2: Net-(LED39-Pad1) -> /led/LRow3
- LR4 pad 1: /led/LRow0 -> Net-(LED4-Pad2)
- LR4 pad 2: Net-(LED4-Pad1) -> /led/LRow0
- LR40 pad 1: /led/LRow0 -> Net-(LED40-Pad2)
- LR40 pad 2: Net-(LED40-Pad1) -> /led/LRow3
- LR41 pad 1: /led/LRow0 -> Net-(LED41-Pad2)
- LR41 pad 2: Net-(LED41-Pad1) -> /led/LRow3
- LR42 pad 1: /led/LRow0 -> Net-(LED42-Pad2)
- LR42 pad 2: Net-(LED42-Pad1) -> /led/LRow3
- LR5 pad 1: /led/LRow0 -> Net-(LED5-Pad2)
- LR5 pad 2: Net-(LED5-Pad1) -> /led/LRow0
- LR6 pad 1: /led/LRow0 -> Net-(LED6-Pad2)
- LR6 pad 2: Net-(LED6-Pad1) -> /led/LRow0
- LR7 pad 1: /led/LRow0 -> Net-(LED7-Pad2)
- LR7 pad 2: Net-(LED7-Pad1) -> /led/LRow0
- LR8 pad 1: /led/LRow0 -> Net-(LED8-Pad2)
- LR8 pad 2: Net-(LED8-Pad1) -> /led/LRow0
- LR9 pad 1: /led/LRow0 -> Net-(LED9-Pad2)
- LR9 pad 2: Net-(LED9-Pad1) -> /led/LRow0
- P1 pad 1: /Col6 -> /GPIO1
- P1 pad 3: /GPIO1 -> /GPIO2
- P2 pad 1: /GPIO3 -> VCC
- P2 pad 2: /GPIO2 -> /GPIO0
- P2 pad 3: /GPIO0 -> /GPIO1
- P2 pad 4: /GPIO1 -> /GPIO2
- P2 pad 5: /GPIO4 -> /GPIO3
- R4 pad 2: /Backlight -> /led/Backlight
- RGBLED1 pad 4: Net-(LR43-Pad1) -> /led/RGB
- SW1 pad 1: /Row0 -> /matrix/Col0
- SW1 pad 2: Net-(D1-Pad2) -> Net-(D1-Pad1)
- SW10 pad 1: /Row0 -> /matrix/Col9
- SW10 pad 2: Net-(D10-Pad2) -> Net-(D10-Pad1)
- SW11 pad 1: /Row0 -> /matrix/Col10
- SW11 pad 2: Net-(D11-Pad2) -> Net-(D11-Pad1)
- SW12 pad 1: /Row1 -> /matrix/Col0
- SW12 pad 2: Net-(D12-Pad2) -> Net-(D12-Pad1)
- SW13 pad 1: /Row1 -> /matrix/Col1
- SW13 pad 2: Net-(D13-Pad2) -> Net-(D13-Pad1)
- SW14 pad 1: /Row1 -> /matrix/Col2
- SW14 pad 2: Net-(D14-Pad2) -> Net-(D14-Pad1)
- SW15 pad 1: /Row1 -> /matrix/Col3
- SW15 pad 2: Net-(D15-Pad2) -> Net-(D15-Pad1)
- SW16 pad 1: /Row1 -> /matrix/Col4
- SW16 pad 2: Net-(D16-Pad2) -> Net-(D16-Pad1)
- SW17 pad 1: /Row1 -> /matrix/Col5
- SW17 pad 2: Net-(D17-Pad2) -> Net-(D17-Pad1)
- SW18 pad 1: /Row1 -> /matrix/Col6
- SW18 pad 2: Net-(D18-Pad2) -> Net-(D18-Pad1)
- SW19 pad 1: /Row1 -> /matrix/Col7
- SW19 pad 2: Net-(D19-Pad2) -> Net-(D19-Pad1)
- SW2 pad 1: /Row0 -> /matrix/Col1
- SW2 pad 2: Net-(D2-Pad2) -> Net-(D2-Pad1)
- SW20 pad 1: /Row1 -> /matrix/Col8
- SW20 pad 2: Net-(D20-Pad2) -> Net-(D20-Pad1)
- SW21 pad 1: /Row1 -> /matrix/Col9
- SW21 pad 2: Net-(D21-Pad2) -> Net-(D21-Pad1)
- SW22 pad 1: /Row1 -> /matrix/Col10
- SW22 pad 2: Net-(D22-Pad2) -> Net-(D22-Pad1)
- SW23 pad 1: /Row2 -> /matrix/Col0
- SW23 pad 2: Net-(D23-Pad2) -> Net-(D23-Pad1)
- SW24 pad 1: /Row2 -> /matrix/Col1
- SW24 pad 2: Net-(D24-Pad2) -> Net-(D24-Pad1)
- SW25 pad 1: /Row2 -> /matrix/Col2
- SW25 pad 2: Net-(D25-Pad2) -> Net-(D25-Pad1)
- SW26 pad 1: /Row2 -> /matrix/Col3
- SW26 pad 2: Net-(D26-Pad2) -> Net-(D26-Pad1)
- SW27 pad 1: /Row2 -> /matrix/Col4
- SW27 pad 2: Net-(D27-Pad2) -> Net-(D27-Pad1)
- SW28 pad 1: /Row2 -> /matrix/Col5
- SW28 pad 2: Net-(D28-Pad2) -> Net-(D28-Pad1)
- SW29 pad 1: /Row2 -> /matrix/Col6
- SW29 pad 2: Net-(D29-Pad2) -> Net-(D29-Pad1)
- SW3 pad 1: /Row0 -> /matrix/Col2
- SW3 pad 2: Net-(D3-Pad2) -> Net-(D3-Pad1)
- SW30 pad 1: /Row2 -> /matrix/Col7
- SW30 pad 2: Net-(D30-Pad2) -> Net-(D30-Pad1)
- SW31 pad 1: /Row2 -> /matrix/Col8
- SW31 pad 2: Net-(D31-Pad2) -> Net-(D31-Pad1)
- SW32 pad 1: /Row2 -> /matrix/Col9
- SW32 pad 2: Net-(D32-Pad2) -> Net-(D32-Pad1)
- SW33 pad 1: /Row2 -> /matrix/Col10
- SW33 pad 2: Net-(D33-Pad2) -> Net-(D33-Pad1)
- SW34 pad 1: /Row3 -> /matrix/Col0
- SW34 pad 2: Net-(D34-Pad2) -> Net-(D34-Pad1)
- SW35 pad 1: /Row3 -> /matrix/Col1
- SW35 pad 2: Net-(D35-Pad2) -> Net-(D35-Pad1)
- SW36 pad 1: /Row3 -> /matrix/Col2
- SW36 pad 2: Net-(D36-Pad2) -> Net-(D36-Pad1)
- SW37 pad 1: /Row3 -> /matrix/Col4
- SW37 pad 2: Net-(D37-Pad2) -> Net-(D37-Pad1)
- SW38 pad 1: /Row3 -> /matrix/Col5
- SW38 pad 2: Net-(D38-Pad2) -> Net-(D38-Pad1)
- SW38_625 pad 1: /Row3 -> /matrix/Col5
- SW38_625 pad 2: Net-(D38-Pad2) -> Net-(D38-Pad1)
- SW38_625 pad HOLE: (no net) -> Net-(D39-Pad1)
- SW39 pad 1: /Row3 -> /matrix/Col7
- SW39 pad 2: Net-(D39-Pad2) -> Net-(D39-Pad1)
- SW4 pad 1: /Row0 -> /matrix/Col3
- SW4 pad 2: Net-(D4-Pad2) -> Net-(D4-Pad1)
- SW40 pad 1: /Row3 -> /matrix/Col8
- SW40 pad 2: Net-(D40-Pad2) -> Net-(D40-Pad1)
- SW41 pad 1: /Row3 -> /matrix/Col9
- SW41 pad 2: Net-(D41-Pad2) -> Net-(D41-Pad1)
- SW42 pad 1: /Row3 -> /matrix/Col10
- SW42 pad 2: Net-(D42-Pad2) -> Net-(D42-Pad1)
- SW5 pad 1: /Row0 -> /matrix/Col4
- SW5 pad 2: Net-(D5-Pad2) -> Net-(D5-Pad1)
- SW6 pad 1: /Row0 -> /matrix/Col5
- SW6 pad 2: Net-(D6-Pad2) -> Net-(D6-Pad1)
- SW7 pad 1: /Row0 -> /matrix/Col6
- SW7 pad 2: Net-(D7-Pad2) -> Net-(D7-Pad1)
- SW8 pad 1: /Row0 -> /matrix/Col7
- SW8 pad 2: Net-(D8-Pad2) -> Net-(D8-Pad1)
- SW9 pad 1: /Row0 -> /matrix/Col8
- SW9 pad 2: Net-(D9-Pad2) -> Net-(D9-Pad1)
- U1 pad 1: /Backlight -> /GPIO4
- U1 pad 11: /Col6 -> /GPIO1
- U1 pad 12: /Col10 -> /matrix/Col6
- U1 pad 18: /GPIO4 -> /GPIO7
- U1 pad 19: /GPIO3 -> /GPIO6
- U1 pad 20: /Row0 -> /matrix/Row0
- U1 pad 21: /Row1 -> /matrix/Row1
- U1 pad 22: /Row3 -> /matrix/Row2
- U1 pad 25: /Row2 -> /GPIO5
- U1 pad 26: /WASD -> /matrix/Row3
- U1 pad 27: /ESC -> /matrix/Col8
- U1 pad 28: /Col7 -> /GPIO3
- U1 pad 29: /Col8 -> /matrix/Col9
- U1 pad 30: /Col9 -> /matrix/Col10
- U1 pad 31: /Caps -> /led/CapsLock
- U1 pad 32: /Bottom -> /led/RGB
- U1 pad 33: Net-(IC1-Pad33) -> GND
- U1 pad 36: /Col5 -> /matrix/Col5
- U1 pad 37: /Col4 -> /matrix/Col4
- U1 pad 38: /Col3 -> /matrix/Col3
- U1 pad 39: /Col2 -> /matrix/Col2
- U1 pad 40: /Col1 -> /matrix/Col1
- U1 pad 41: /Col0 -> /matrix/Col0
- U1 pad 8: /GPIO2 -> /matrix/Col7
- U1 pad 9: /GPIO1 -> /GPIO2
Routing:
- net /led/LRow0: track 829.8 -> 192.9 mm, vias 37 -> 0
- net /matrix/Row3: track 0.00 -> 340.4 mm, vias 0 -> 6
- net GND: track 1090.7 -> 767.0 mm, vias 15 -> 13
- net /led/LRow3: track 0.00 -> 295.9 mm, vias 0 -> 4
- net /matrix/Row0: track 0.00 -> 277.5 mm, vias 0 -> 2
- net /matrix/Row1: track 0.00 -> 266.3 mm, vias 0 -> 2
- net /matrix/Row2: track 0.00 -> 244.5 mm, vias 0 -> 2
- net /WASD: track 243.4 -> 0.00 mm, vias 2 -> 0
- net /GPIO6: track 0.00 -> 239.6 mm, vias 0 -> 3
- net /Row3: track 224.3 -> 0.00 mm
- net /led/LVCC: track 0.00 -> 220.5 mm, vias 0 -> 4
- net /matrix/Col0: track 0.00 -> 215.5 mm, vias 0 -> 3
- net /ESC: track 203.0 -> 0.00 mm, vias 2 -> 0
- net /led/LRow1: track 0.00 -> 201.1 mm
- net /led/LRow2: track 0.00 -> 200.9 mm
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- added copper zone on B.Cu, net /SHIELD
- added copper zone on F.Cu, net /SHIELD
- removed copper zone on B.Cu, net (none)
- removed copper zone on F.Cu, net (none)
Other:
- board size 228.6 x 76.2 mm -> 229.6 x 77.2 mm
- net class Default: clearance 0.2 -> 0.127; trace_width 0.25 -> 0.4064; via_drill 0.4 -> 0.3
- net class Minimum added: clearance 0.127, trace_width 0.254, via_dia 0.6, via_drill 0.3
- net class Power added: clearance 0.127, trace_width 0.6096, via_dia 0.6, via_drill 0.3
- rule pad_to_mask_clearance: 0.2 -> 0.1
- rule trace_clearance: 0.2 -> 0.127
- rule trace_min: 0.25 -> 0.1524
- rule via_min_size: 0.6 -> 0.599999
- board text added: "/RESET"
- board text added: "GND"
- board text added: "MISO"
- board text added: "MOSI"
- board text added: "PB4"
- board text added: "PD4"
- board text added: "PE6"
- board text added: "SCK"
- board text added: "SCL"
- board text added: "SDA"
- board text added: "VCC"
- board text added: "v0.3"
- board text added: "©2017 K.T.E.C."
- board text removed: "Daisy"
- board text removed: "Designed by hging K.T.E.C. presents"
- board text removed: "v0.1a"
